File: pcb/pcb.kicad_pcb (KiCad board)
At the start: 2 copper layers, 77.3 x 67 mm, 45 parts, among them CN1 Battery_Cell, Q1 AO3401A, Q2 AO3400A, U1 TPS63802DLAT, U2 USB-C 6PIN, U3 BQ24075RGTR, U4 ESP-32S DevBoard, U5 Water_Sensor, U6 Pump

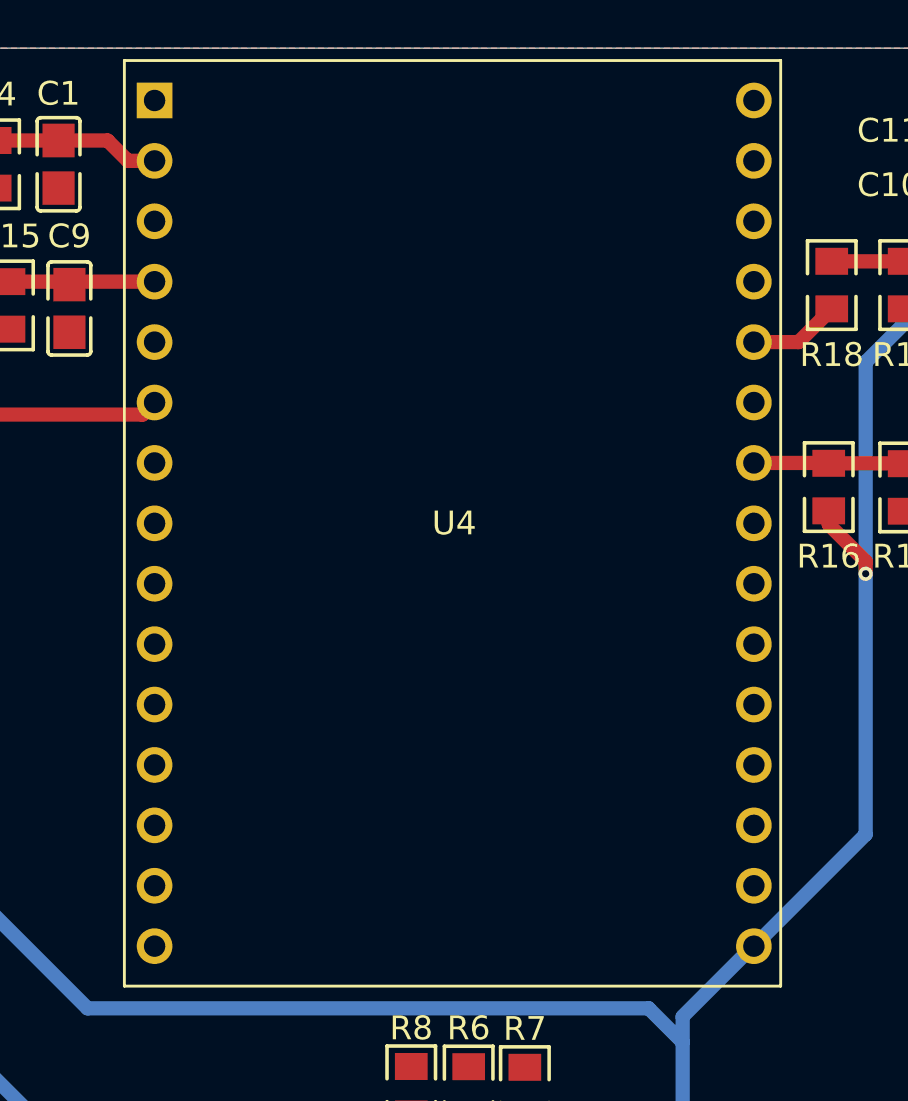
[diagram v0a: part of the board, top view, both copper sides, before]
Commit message: Added some more symbol information
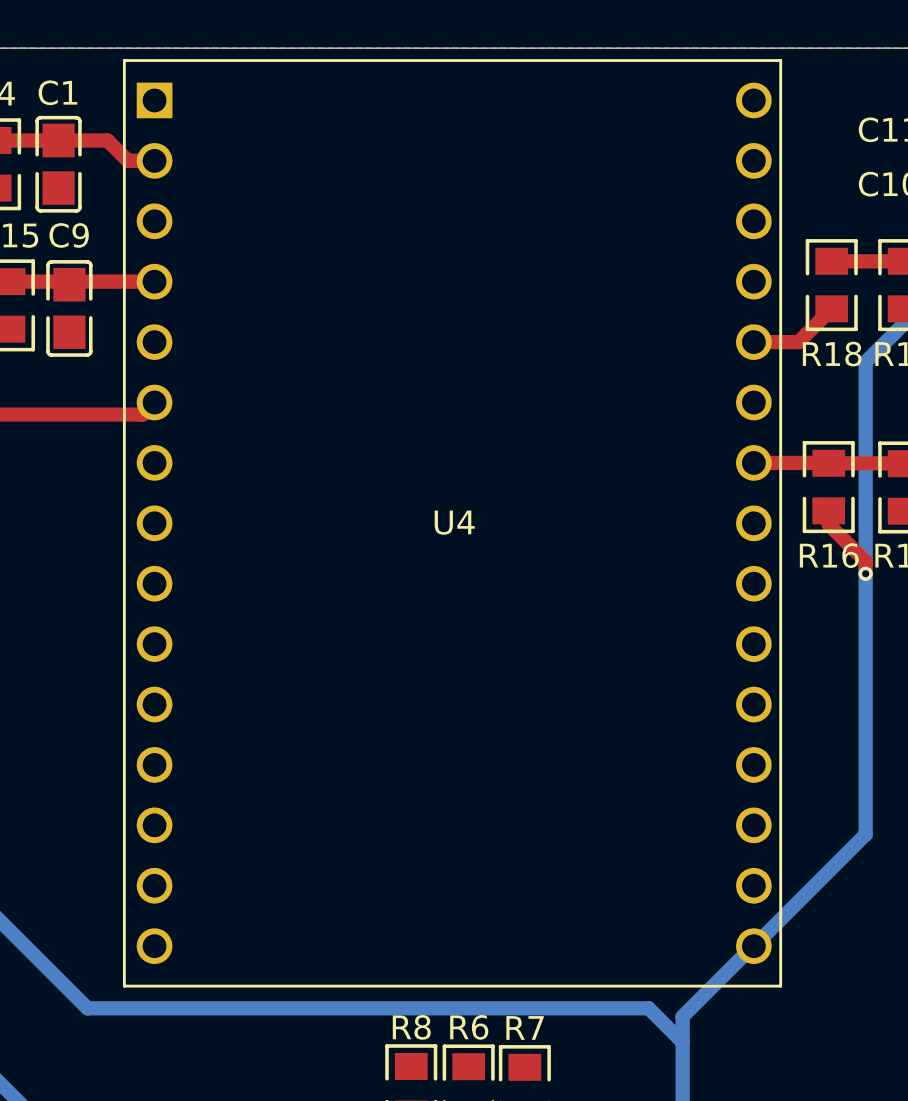
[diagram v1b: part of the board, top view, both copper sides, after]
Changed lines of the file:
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@@
 			(at 0 0)
 			(size 1.5 1.5)
-			(drill 0.9)
+			(drill 1.0)
 			(layers "*.Cu" "*.Mask")
 			(remove_unused_layers yes)
@@
 			(at 0 2.54)
 			(size 1.5 1.5)
-			(drill 0.9)
+			(drill 1.0)
 			(layers "*.Cu" "*.Mask")
 			(remove_unused_layers yes)
@@
 			(at 0 5.08)
 			(size 1.5 1.5)
-			(drill 0.9)
+			(drill 1.0)
 			(layers "*.Cu" "*.Mask")
 			(remove_unused_layers yes)
@@
 			(at 0 7.62)
 			(size 1.5 1.5)
-			(drill 0.9)
+			(drill 1.0)
 			(layers "*.Cu" "*.Mask")
 			(remove_unused_layers yes)
@@
 			(at 0 10.16)
 			(size 1.5 1.5)
-			(drill 0.9)
+			(drill 1.0)
 			(layers "*.Cu" "*.Mask")
 			(remove_unused_layers yes)
@@
 			(at 0 12.7)
 			(size 1.5 1.5)
-			(drill 0.9)
+			(drill 1.0)
 			(layers "*.Cu" "*.Mask")
 			(remove_unused_layers yes)
@@
 			(at 0 15.24)
 			(size 1.5 1.5)
-			(drill 0.9)
+			(drill 1.0)
 			(layers "*.Cu" "*.Mask")
 			(remove_unused_layers yes)
@@
 			(at 0 17.78)
 			(size 1.5 1.5)
-			(drill 0.9)
+			(drill 1.0)
 			(layers "*.Cu" "*.Mask")
 			(remove_unused_layers yes)
@@
 			(at 0 20.32)
 			(size 1.5 1.5)
-			(drill 0.9)
+			(drill 1.0)
 			(layers "*.Cu" "*.Mask")
 			(remove_unused_layers yes)
@@
 			(at 0 22.86)
 			(size 1.5 1.5)
-			(drill 0.9)
+			(drill 1.0)
 			(layers "*.Cu" "*.Mask")
 			(remove_unused_layers yes)
@@
 			(at 0 25.4)
 			(size 1.5 1.5)
-			(drill 0.9)
+			(drill 1.0)
 			(layers "*.Cu" "*.Mask")
 			(remove_unused_layers yes)
@@
 			(at 0 27.94)
 			(size 1.5 1.5)
-			(drill 0.9)
+			(drill 1.0)
 			(layers "*.Cu" "*.Mask")
 			(remove_unused_layers yes)
@@
 			(at 0 30.48)
 			(size 1.5 1.5)
-			(drill 0.9)
+			(drill 1.0)
 			(layers "*.Cu" "*.Mask")
 			(remove_unused_layers yes)
@@
 			(at 0 33.02)
 			(size 1.5 1.5)
-			(drill 0.9)
+			(drill 1.0)
 			(layers "*.Cu" "*.Mask")
 			(remove_unused_layers yes)
@@
 			(at 0 35.56)
 			(size 1.5 1.5)
-			(drill 0.9)
+			(drill 1.0)
 			(layers "*.Cu" "*.Mask")
 			(remove_unused_layers yes)
@@
 			(at 25.2 0)
 			(size 1.5 1.5)
-			(drill 0.9)
+			(drill 1.0)
 			(layers "*.Cu" "*.Mask")
 			(remove_unused_layers yes)
@@
 			(at 25.2 2.54)
 			(size 1.5 1.5)
-			(drill 0.9)
+			(drill 1.0)
 			(layers "*.Cu" "*.Mask")
 			(remove_unused_layers yes)
@@
 			(at 25.2 5.08)
 			(size 1.5 1.5)
-			(drill 0.9)
+			(drill 1.0)
 			(layers "*.Cu" "*.Mask")
 			(remove_unused_layers yes)
@@
 			(at 25.2 7.62)
 			(size 1.5 1.5)
-			(drill 0.9)
+			(drill 1.0)
 			(layers "*.Cu" "*.Mask")
 			(remove_unused_layers yes)
@@
 			(at 25.2 10.16)
 			(size 1.5 1.5)
-			(drill 0.9)
+			(drill 1.0)
 			(layers "*.Cu" "*.Mask")
 			(remove_unused_layers yes)
@@
 			(at 25.2 12.7)
 			(size 1.5 1.5)
-			(drill 0.9)
+			(drill 1.0)
 			(layers "*.Cu" "*.Mask")
 			(remove_unused_layers yes)
@@
 			(at 25.2 15.24)
 			(size 1.5 1.5)
-			(drill 0.9)
+			(drill 1.0)
 			(layers "*.Cu" "*.Mask")
 			(remove_unused_layers yes)
@@
 			(at 25.2 17.78)
 			(size 1.5 1.5)
-			(drill 0.9)
+			(drill 1.0)
 			(layers "*.Cu" "*.Mask")
 			(remove_unused_layers yes)
@@
 			(at 25.2 20.32)
 			(size 1.5 1.5)
-			(drill 0.9)
+			(drill 1.0)
 			(layers "*.Cu" "*.Mask")
 			(remove_unused_layers yes)
@@
 			(at 25.2 22.86)
 			(size 1.5 1.5)
-			(drill 0.9)
+			(drill 1.0)
 			(layers "*.Cu" "*.Mask")
 			(remove_unused_layers yes)
@@
 			(at 25.2 25.4)
 			(size 1.5 1.5)
-			(drill 0.9)
+			(drill 1.0)
 			(layers "*.Cu" "*.Mask")
 			(remove_unused_layers yes)
@@
 			(at 25.2 27.94)
 			(size 1.5 1.5)
-			(drill 0.9)
+			(drill 1.0)
 			(layers "*.Cu" "*.Mask")
 			(remove_unused_layers yes)
@@
 			(at 25.2 30.48)
 			(size 1.5 1.5)
-			(drill 0.9)
+			(drill 1.0)
 			(layers "*.Cu" "*.Mask")
 			(remove_unused_layers yes)
@@
 			(at 25.2 33.02)
 			(size 1.5 1.5)
-			(drill 0.9)
+			(drill 1.0)
 			(layers "*.Cu" "*.Mask")
 			(remove_unused_layers yes)
@@
 			(at 25.2 35.56)
 			(size 1.5 1.5)
-			(drill 0.9)
-			(layers "*.Cu" "*.Mask")
-			(remove_unused_layers yes)
+			(drill 1.0)
+			(layers "*.Cu" "*.Mask")
+			(remove_unused_layers yes)
